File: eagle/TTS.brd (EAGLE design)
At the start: 35.2 x 26.7 mm, 14 parts, among them IC1 LM386N-1

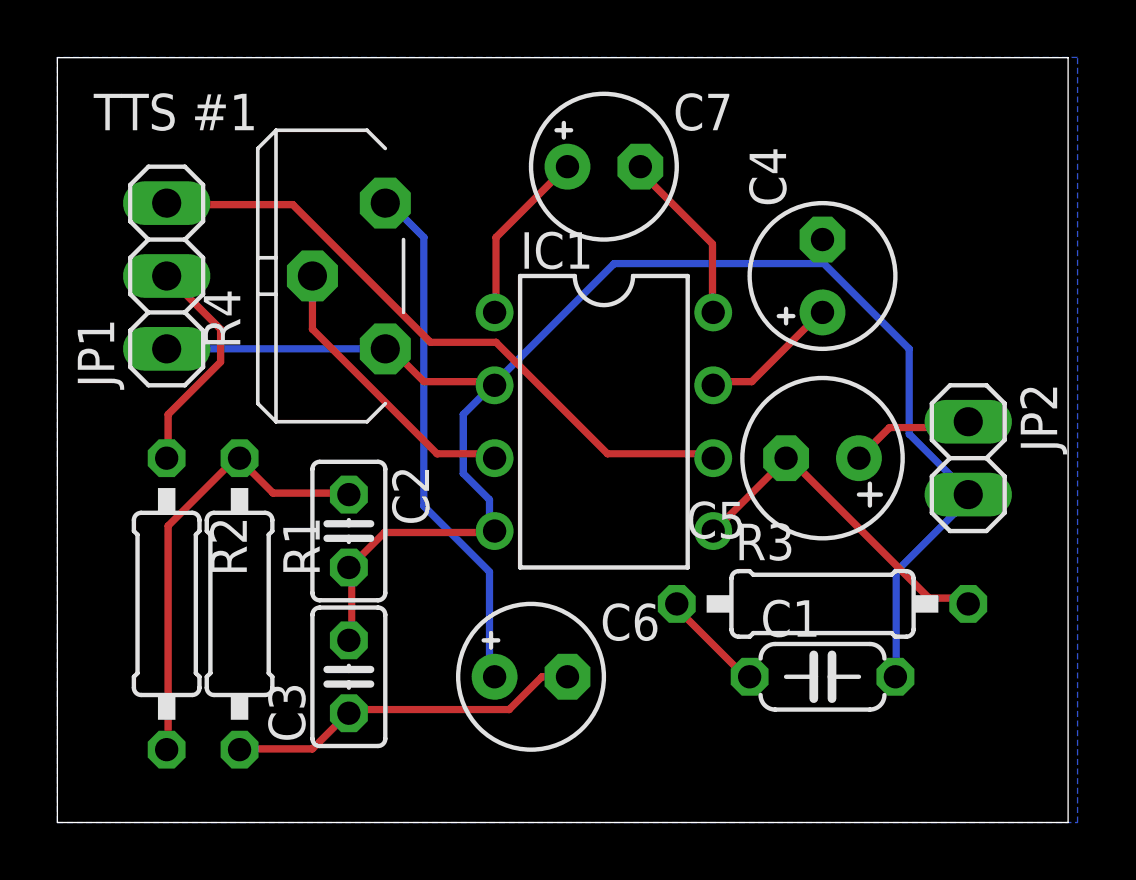
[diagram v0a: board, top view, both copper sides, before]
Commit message: updates after build #1
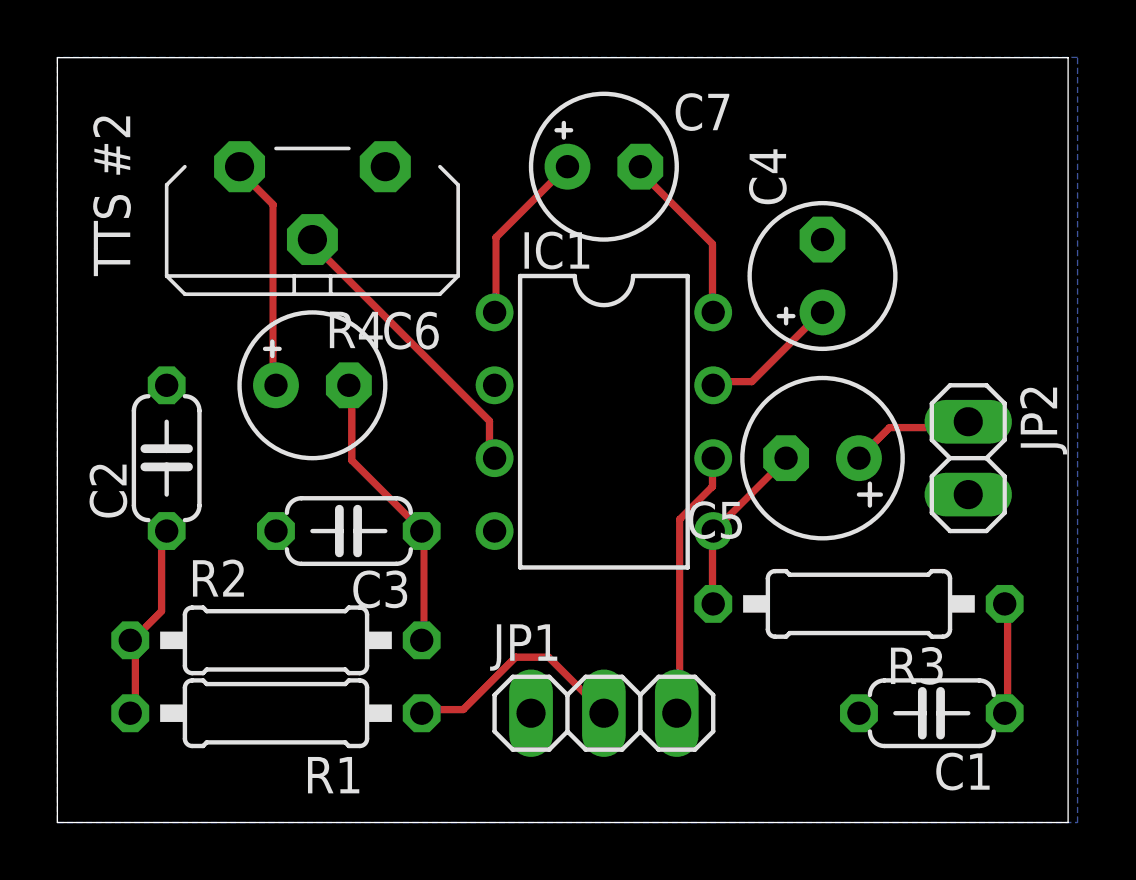
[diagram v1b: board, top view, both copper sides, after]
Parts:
- C2, C3: device resistor:C025-025X050 -> rcl:C050-024X044
- R3: value 10k -> 10R
- moved JP1 21.6 mm to (44.5, 33.0), turned to 0 degrees
- moved C6 12.7 mm to (34.3, 44.5)
- moved C2 6.84 mm to (29.2, 41.9), turned to 90 degrees
- moved C3 5.08 mm to (35.6, 39.4), turned to 180 degrees
- moved C1 4.02 mm to (55.9, 33.0), turned to 180 degrees
- moved R2 4.02 mm to (33.0, 35.6), turned to 0 degrees
- moved R1 4.02 mm to (33.0, 33.0), turned to 180 degrees
- moved R4 2.84 mm to (34.3, 50.8), turned to 180 degrees
- moved R3 1.27 mm to (53.3, 36.8), turned to 180 degrees
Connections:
- net N$2: now also R1.2, R2.1; no longer R1.1, R2.2
- net N$3: now also R2.2; no longer R1.2
- net N$7: now also R1.1; no longer R2.1
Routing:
- net GND: track 57.8 -> 0.00 mm
- net VCC: track 22.8 -> 9.40 mm
- net N$9: track 18.3 -> 8.13 mm
- net N$2: track 15.6 -> 7.15 mm
- net N$5: track 12.2 -> 6.14 mm
- net N$3: track 12.5 -> 10.0 mm
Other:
- board text added: "TTS #2"
- board text removed: "TTS #1"
